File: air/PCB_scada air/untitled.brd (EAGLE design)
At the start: 80 x 80 mm, 55 parts, among them J1 10118193-0001LF, K1 351, Q1 MMBT3904, Q2 MMBT3904, Q3 12MHz, Q4 S9013, U1 CH340G, U2 ESP32-WROOM-32D, U3 AMS1117, U4 ADS1115IDGSR, U5 PC817X2NIP0F, X1 MSTBA2, X2 MSTBA3, X3 MSTBA4, X4 MSTBA5

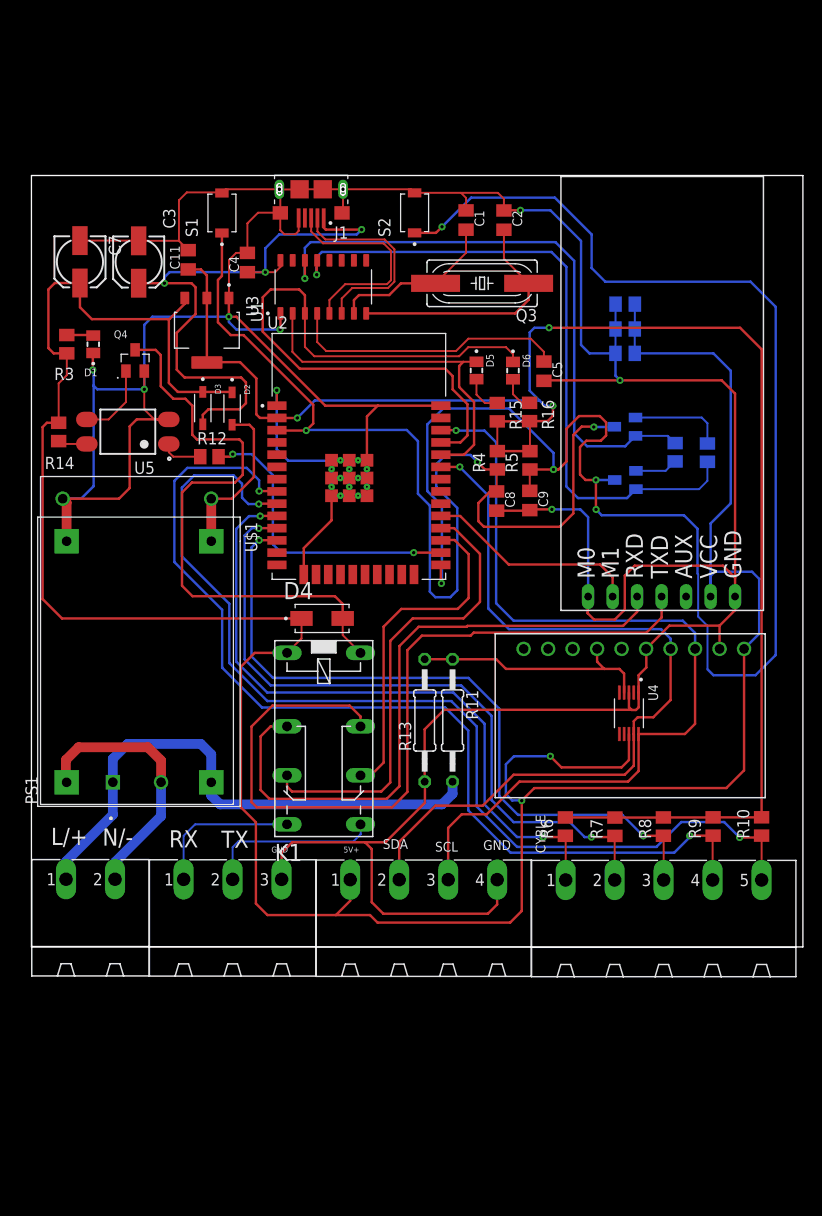
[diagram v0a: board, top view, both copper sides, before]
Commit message: revisi scada air
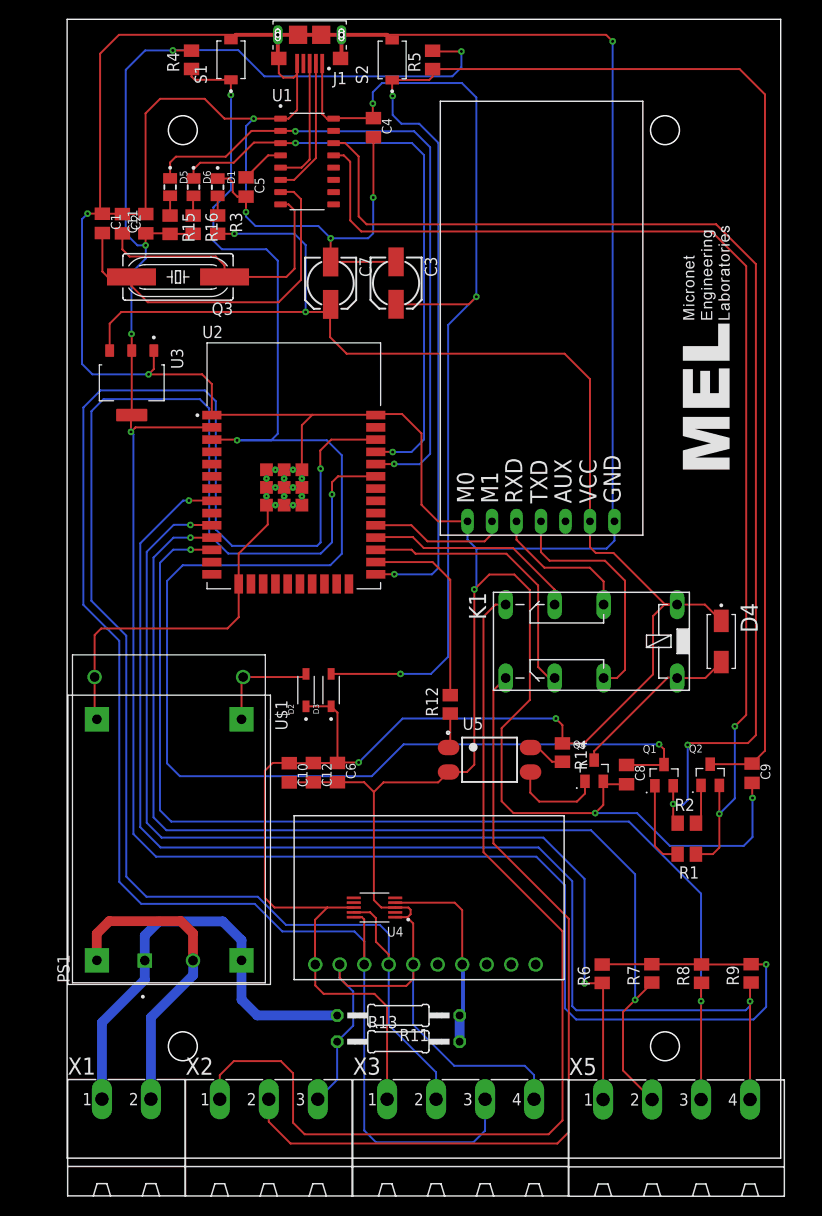
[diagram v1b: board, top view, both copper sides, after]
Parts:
- removed R10: (no value), rcl:M0805
- removed X4: MSTBA5, con-phoenix-508:MSTBA5
- added X5: MSTBA4, con-phoenix-508:MSTBA4
- moved Q4 63.8 mm to (58.4, 38.3)
- moved R14 61.9 mm to (55.1, 40.2)
- moved C10 59.8 mm to (26.7, 38.1), flipped to the top, turned to 270 degrees
- moved C6 54.8 mm to (31.7, 38.1), flipped to the top, turned to 270 degrees
- moved C12 54.2 mm to (29.2, 38.1), flipped to the top, turned to 270 degrees
- moved R4 52.3 mm to (16.6, 112.0)
- moved U5 50.6 mm to (47.5, 39.4), turned to 0 degrees
- moved R5 42.7 mm to (41.6, 112.0)
- moved R1 41.7 mm to (68.0, 29.6), flipped to the top, turned to 180 degrees
- moved D4 41.5 mm to (71.5, 51.7), turned to 270 degrees
- moved R16 39.9 mm to (16.8, 94.9)
- moved C2 39.6 mm to (9.43, 95.0)
- moved R15 39.1 mm to (14.4, 94.9)
- moved R2 38.5 mm to (68.0, 32.8), flipped to the top, turned to 0 degrees
- moved D6 38.2 mm to (16.8, 98.8)
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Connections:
- removed net CYBLE5: R10.1, U2.9, X4.5
- net CYBLE1: now also X5.1; no longer X4.1
- net CYBLE2: now also X5.2; no longer X4.2
- net CYBLE3: now also X5.3; no longer X4.3
- net CYBLE4: now also X5.4; no longer X4.4
- net VCC: no longer R10.2
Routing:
- net GND: track 441.4 -> 564.8 mm, vias 8 -> 10
- net CYBLE5: track 107.1 -> 0.00 mm, vias 2 -> 0
- net RXLORA_CONFIG: track 15.7 -> 103.8 mm
- net SCL: track 92.0 -> 176.7 mm
- net SDA: track 85.3 -> 157.8 mm
- net VCC: track 170.9 -> 243.2 mm, vias 3 -> 6
- net TXLORA_CONFIG: track 18.2 -> 85.7 mm
- net OUT+: track 289.1 -> 224.5 mm, vias 2 -> 4
- net EN: track 111.9 -> 174.2 mm
- net TX_LORA: track 83.2 -> 25.0 mm
- net RTS: track 63.7 -> 120.5 mm, vias 1 -> 2
- net RX_LORA: track 66.3 -> 15.1 mm
- net DTR: track 70.7 -> 118.2 mm, vias 1 -> 2
- net N$13: track 62.1 -> 18.1 mm
- net CYBLE2: track 72.3 -> 113.9 mm
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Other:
- board size 80 x 80 mm -> 74 x 118.1 mm
- board text removed: "5V+"
- board text removed: "CYBLE"
- board text removed: "GND"
- board text removed: "L/+"
- board text removed: "N/-"
- board text removed: "RX"
- board text removed: "SCL"
- board text removed: "SDA"
- board text removed: "TX"
